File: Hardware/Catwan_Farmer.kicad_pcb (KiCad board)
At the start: 2 copper layers, 60 x 70 mm, 56 parts, among them J1 SENSOR 1, J10 VSP, J2 SENSOR 2, J3 SENSOR 3, J4 BATT, J5 USB_B, J6 Conn_01x04, J7 DHT22, J9 SENSOR 4, SW1 SW_Push, U1 AP2114N-1.0, U2 RFM95W-915S2, U3 ATSAMD21E18A-MU, U4 MCP73831-4-OT, U5 74HC4052, Y1 32.768Khz

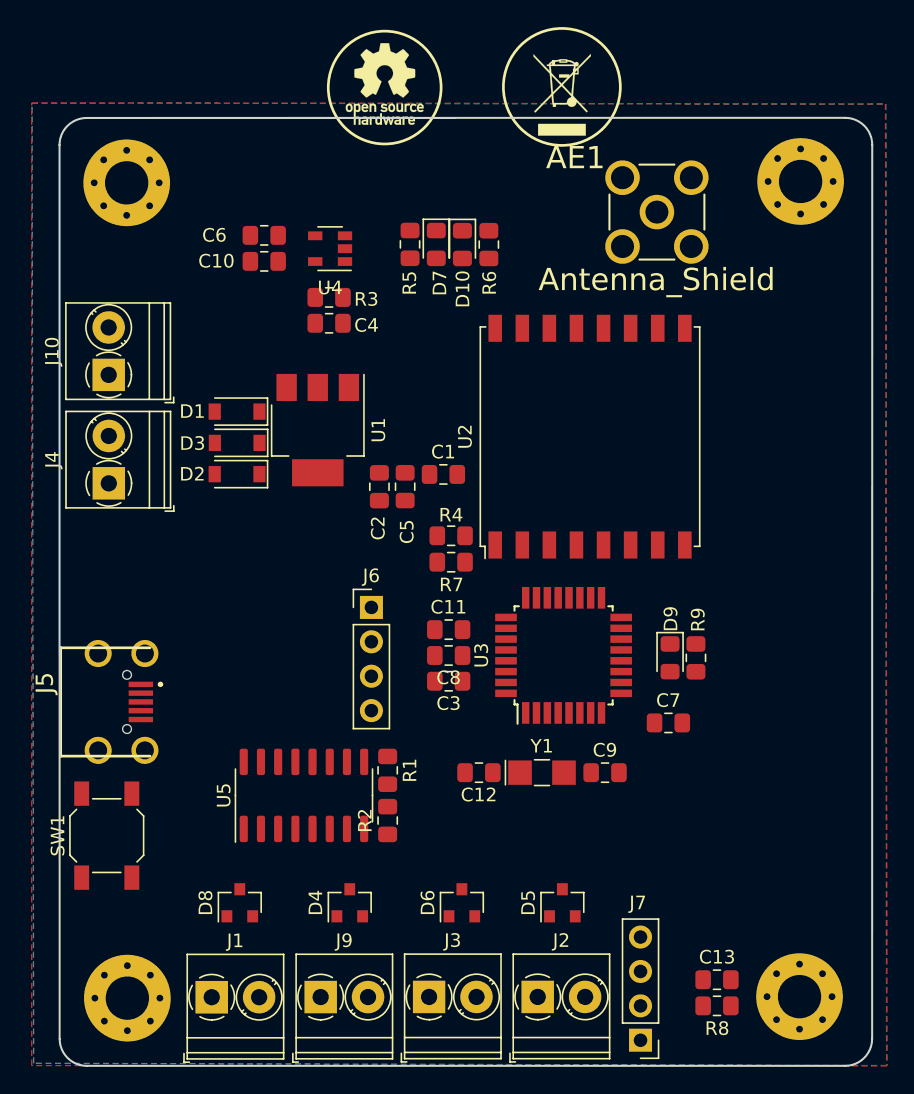
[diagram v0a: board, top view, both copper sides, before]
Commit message: 7HC40 and Diodes
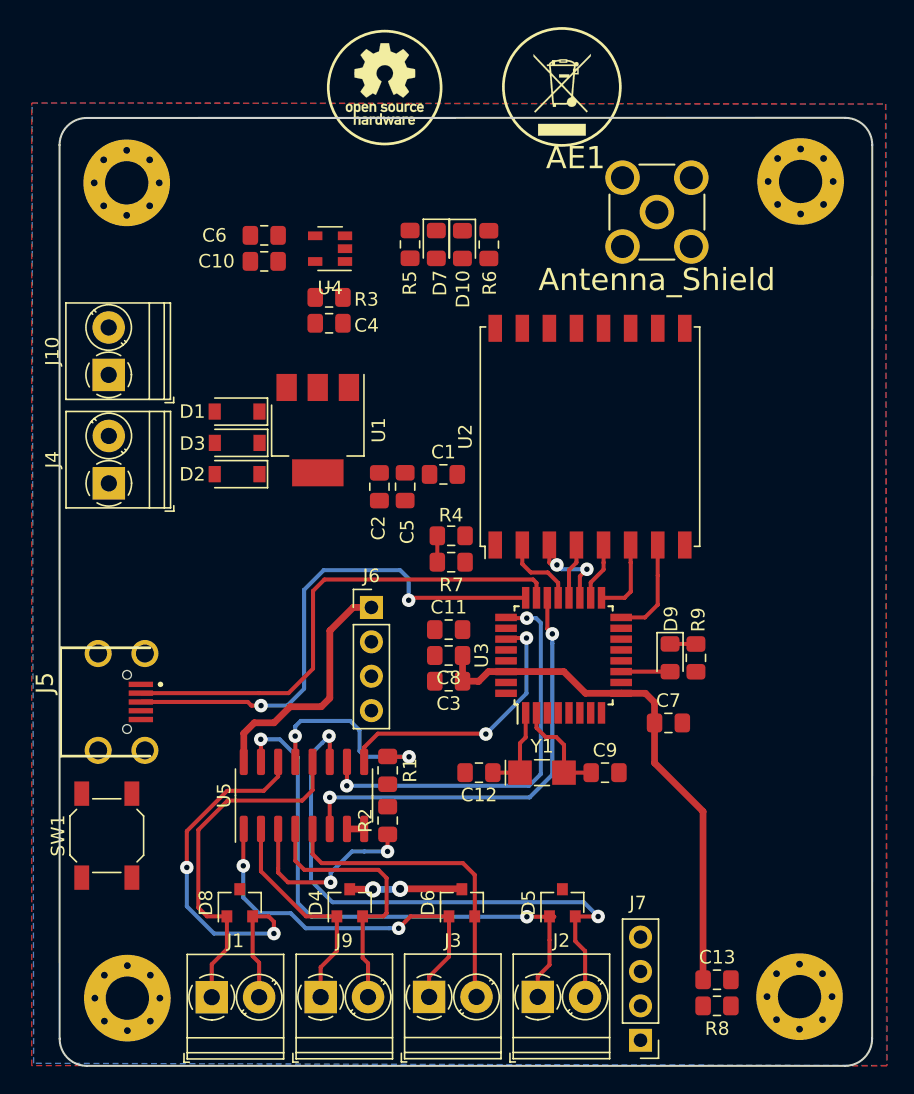
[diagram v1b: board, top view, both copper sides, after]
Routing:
- net +3V3: track 0.00 -> 57.6 mm
- net Net-(D5-Pad2): track 0.00 -> 43.4 mm, vias 0 -> 2
- net Net-(D5-Pad1): track 0.00 -> 41.7 mm, vias 0 -> 2
- net /D+: track 0.00 -> 38.9 mm, vias 0 -> 2
- net /D-: track 0.00 -> 37.3 mm
- net /EN: track 0.00 -> 32.7 mm, vias 0 -> 2
- net Net-(D8-Pad2): track 0.00 -> 31.1 mm, vias 0 -> 2
- net /S0: track 0.00 -> 30.4 mm, vias 0 -> 2
- net Net-(D6-Pad1): track 0.00 -> 28.1 mm, vias 0 -> 2
- net Net-(D8-Pad1): track 0.00 -> 26.3 mm
- net Net-(D6-Pad2): track 0.00 -> 23.5 mm
- net /S1: track 0.00 -> 20.4 mm, vias 0 -> 2
- net Net-(D4-Pad2): track 0.00 -> 20.2 mm
- net Net-(D4-Pad1): track 0.00 -> 16.6 mm
- net /SENS_X: track 0.00 -> 14.8 mm, vias 0 -> 2
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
